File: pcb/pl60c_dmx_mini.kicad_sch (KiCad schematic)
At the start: 36 parts, among them J1 USB-C 16P, J2 XLR-5 female (DMX OUT), Q1 S8050, SW2 BOOT, SW3 USER, U1 ESP32-S3-MINI-1-N8, U2 AP2112K-3.3, U3 SP3485EN, U4 USBLC6-2SC6

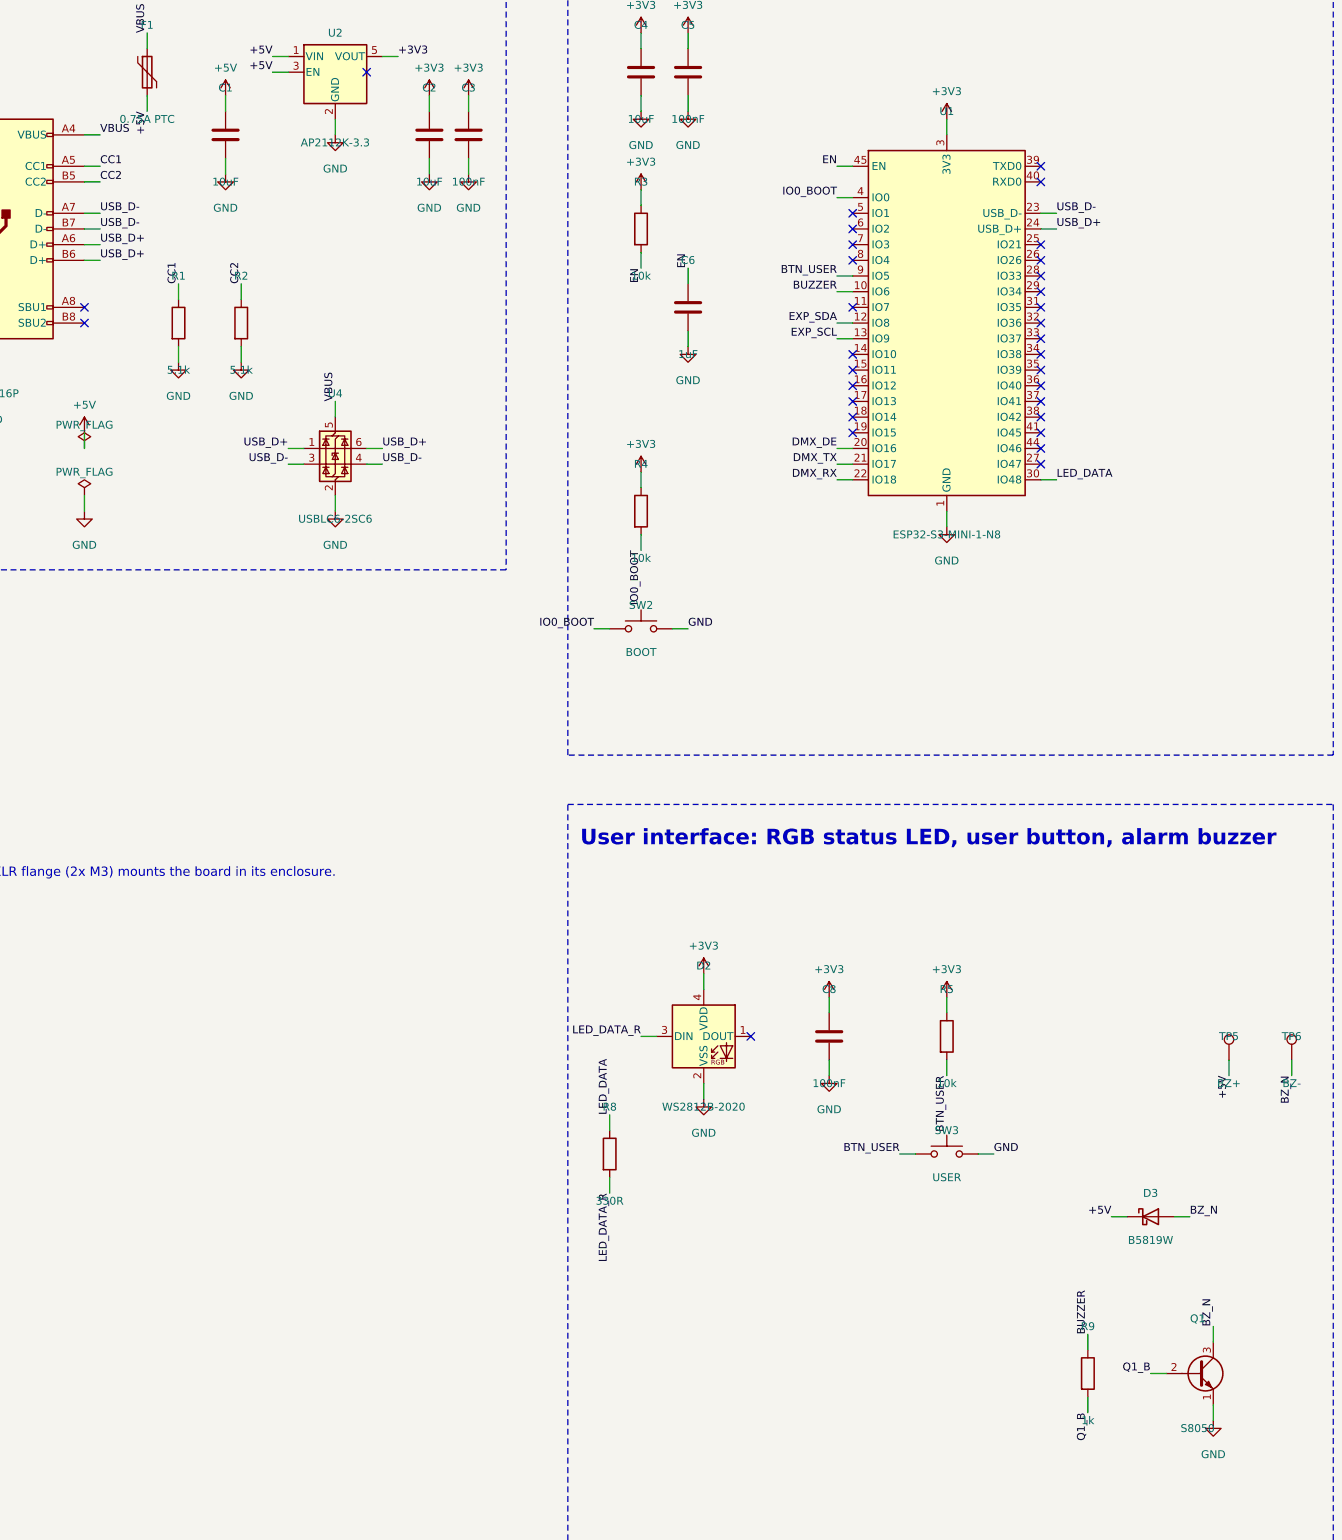
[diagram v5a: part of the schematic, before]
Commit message: auto: 2026-09-02 14:45:57
Co-Authored-By: Claude Fable 5.1 <noreply@anthropic.com>
Claude-Session: https://claude.ai/code/session_01WsrVZb94LwbHVAmBvsSTfn
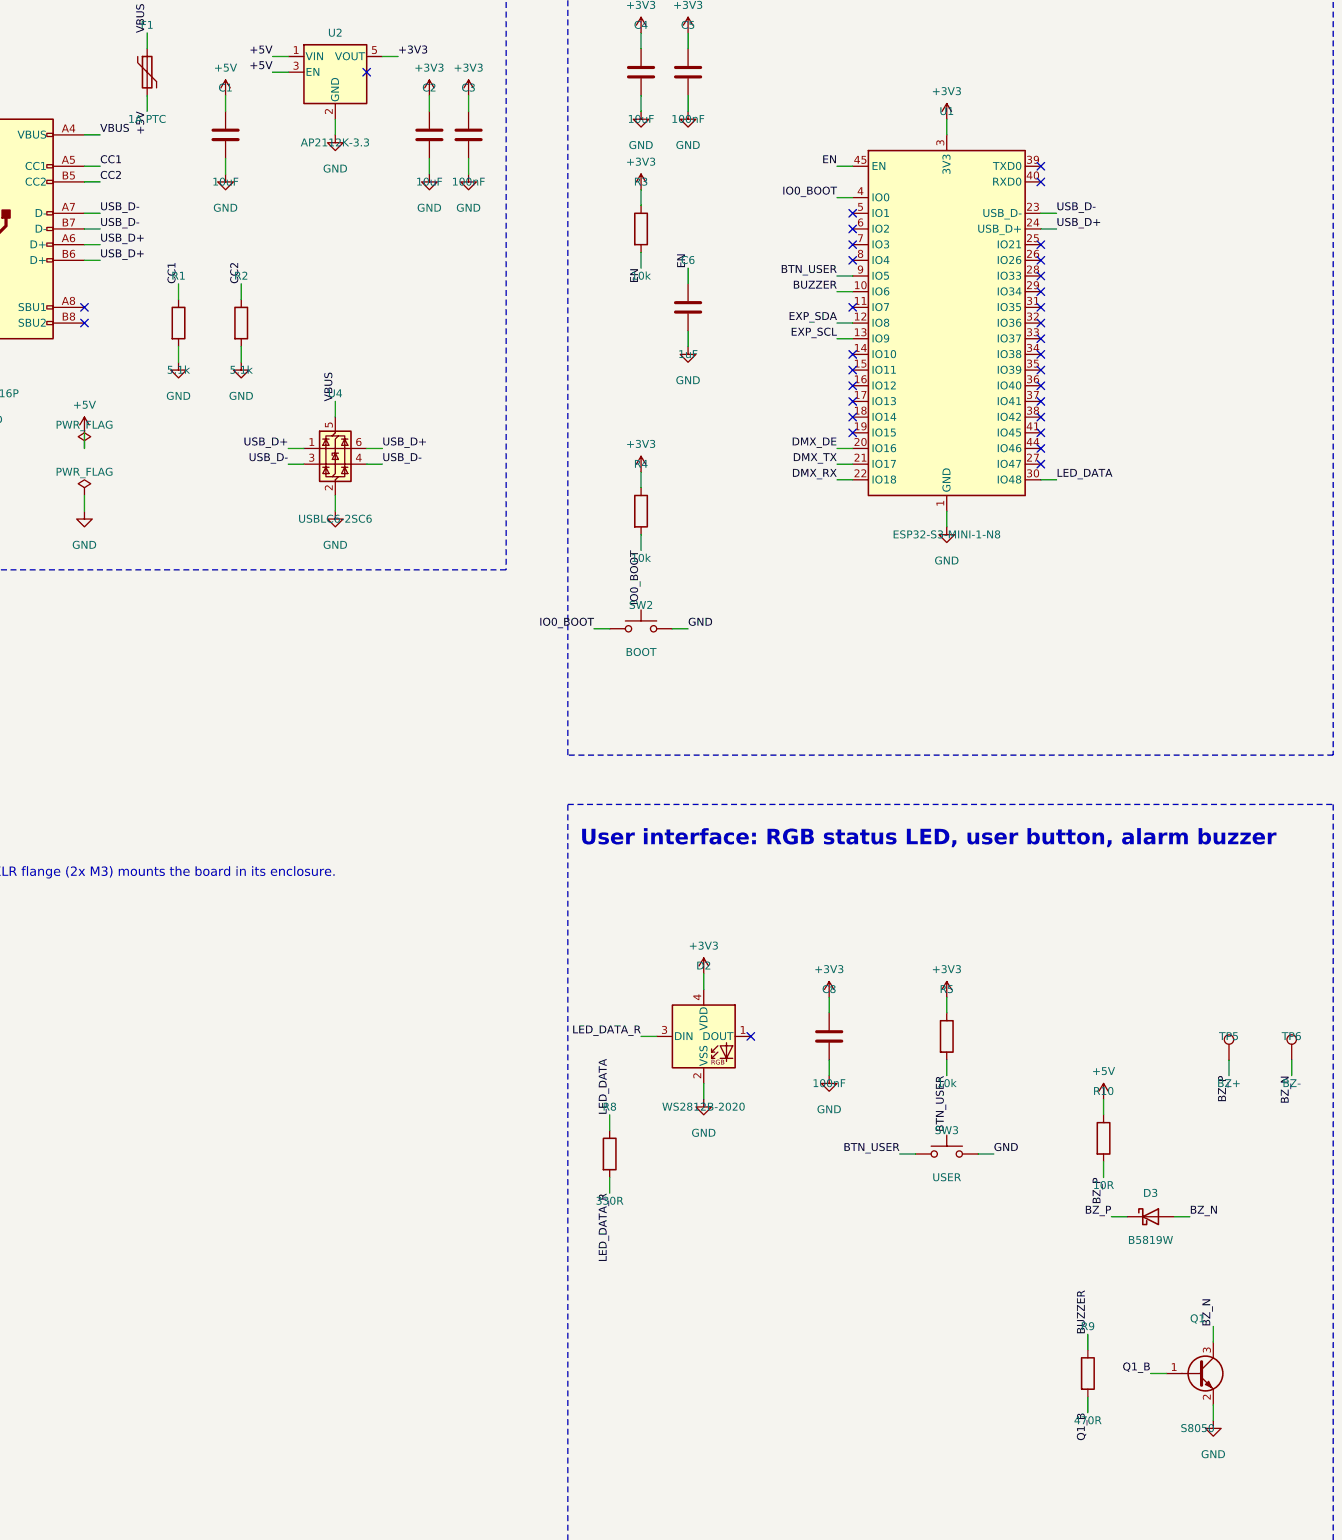
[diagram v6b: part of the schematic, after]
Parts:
- added R10: 10R, Resistor_SMD:R_1206_3216Metric, symbol Device:R
- F1: value 0.75A PTC -> 1A PTC; footprint Fuse:Fuse_0805_2012Metric -> Fuse:Fuse_1206_3216Metric; LCSC C7472571 -> C5358568; MPN 0805L075/6AR -> BSMD1206-100-30V
- Q1: symbol Transistor_BJT:S8050 -> Transistor_BJT:BC817
- R9: value 1k -> 470R; LCSC C11702 -> C25117
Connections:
- net +5V: now also R10.1; no longer D3.1 (K), TP5.1
- net GND: now also Q1.2 (E); no longer Q1.1 (E)
- net Q1_B: now also Q1.1 (B); no longer Q1.2 (B)
- new net BZ_P: D3.1 (K), R10.2, TP5.1
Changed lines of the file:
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@@
 			)
 		)
-		(property "Value" "0.75A PTC"
+		(property "Value" "1A PTC"
 			(at 69.85 46.99 0)
 			(effects
@@
 			)
 		)
-		(property "Footprint" "Fuse:Fuse_0805_2012Metric"
+		(property "Footprint" "Fuse:Fuse_1206_3216Metric"
 			(at 69.85 39.37 0)
 			(effects
@@
 			)
 		)
-		(property "Description" "PTC resettable fuse 0805, 0.75 A hold, 6 V"
+		(property "Description" "PTC resettable fuse 1206, 1 A hold / 1.8 A trip"
 			(at 69.85 39.37 0)
 			(effects
@@
 			)
 		)
-		(property "LCSC" "C7472571"
+		(property "LCSC" "C5358568"
 			(at 69.85 39.37 0)
 			(effects
@@
 			)
 		)
-		(property "MPN" "0805L075/6AR"
+		(property "MPN" "BSMD1206-100-30V"
 			(at 69.85 39.37 0)
 			(effects
@@
 			)
 		)
-		(property "Value" "1k"
+		(property "Value" "470R"
 			(at 222.25 257.81 0)
 			(effects
@@
 			)
 		)
-		(property "Description" "1k 0402"
+		(property "Description" "470R 0402 base resistor"
 			(at 222.25 250.19 0)
 			(effects
@@
 			)
 		)
-		(property "LCSC" "C11702"
+		(property "LCSC" "C25117"
 			(at 222.25 250.19 0)
 			(effects
@@
 	)
 	(symbol
-		(lib_id "Transistor_BJT:S8050")
+		(lib_id "Transistor_BJT:BC817")
 		(at 240.03 250.19 0)
 		(unit 1)
@@
 	(wire
 		(pts
+			(xy 234.95 250.19)
+			(xy 232.41 250.19)
+		)
+		(stroke
+			(width 0)
+			(type default)
+		)
+	)
+	(label "Q1_B"
+		(at 232.41 250.19 180)
+		(fields_autoplaced yes)
+		(effects
+			(font
+				(size 1.27 1.27)
+			)
+			(justify right bottom)
+		)
+	)
+	(wire
+		(pts
 			(xy 242.57 255.27)
 			(xy 242.57 257.81)
@@
 	(wire
 		(pts
-			(xy 234.95 250.19)
-			(xy 232.41 250.19)
-		)
-		(stroke
-			(width 0)
-			(type default)
-		)
-	)
-	(label "Q1_B"
-		(at 232.41 250.19 180)
-		(fields_autoplaced yes)
-		(effects
-			(font
-				(size 1.27 1.27)
-			)
-			(justify right bottom)
-		)
-	)
-	(wire
-		(pts
 			(xy 242.57 245.11)
 			(xy 242.57 242.57)
@@
 		)
 	)
-	(label "+5V"
+	(label "BZ_P"
 		(at 226.06 224.79 180)
 		(fields_autoplaced yes)
@@
 	)
 	(symbol
+		(lib_id "Device:R")
+		(at 224.79 212.09 0)
+		(unit 1)
+		(exclude_from_sim no)
+		(in_bom yes)
+		(on_board yes)
+		(dnp no)
+		(property "Reference" "R10"
+			(at 224.79 204.47 0)
+			(effects
+				(font
+					(size 1.27 1.27)
+				)
+			)
+		)
+		(property "Value" "10R"
+			(at 224.79 219.71 0)
+			(effects
+				(font
+					(size 1.27 1.27)
+				)
+			)
+		)
+		(property "Footprint" "Resistor_SMD:R_1206_3216Metric"
+			(at 224.79 212.09 0)
+			(effects
+				(font
+					(size 1.27 1.27)
+				)
+				(hide yes)
+			)
+		)
+		(property "Datasheet" "~"
+			(at 224.79 212.09 0)
+			(effects
+				(font
+					(size 1.27 1.27)
+				)
+				(hide yes)
+			)
+		)
+		(property "Description" "10R 1206 250mW buzzer series resistor"
+			(at 224.79 212.09 0)
+			(effects
+				(font
+					(size 1.27 1.27)
+				)
+				(hide yes)
+			)
+		)
+		(property "LCSC" "C17903"
+			(at 224.79 212.09 0)
+			(effects
+				(font
+					(size 1.27 1.27)
+				)
+				(hide yes)
+			)
+		)
+		(pin "1"
+		)
+		(pin "2"
+		)
+		(instances
+			(project "pl60c_dmx_mini"
+				(path "/e63f84e3-7254-5f79-8caa-7afae8cc707c"
+					(reference "R10")
+					(unit 1)
+				)
+			)
+		)
+	)
+	(wire
+		(pts
+			(xy 224.79 208.28)
+			(xy 224.79 205.74)
+		)
+		(stroke
+			(width 0)
+			(type default)
+		)
+	)
+	(symbol
+		(lib_id "power:+5V")
+		(at 224.79 205.74 0)
+		(unit 1)
+		(exclude_from_sim no)
+		(in_bom yes)
+		(on_board yes)
+		(dnp no)
+		(property "Reference" "#PWR034"
+			(at 224.79 205.74 0)
+			(effects
+				(font
+					(size 1.27 1.27)
+				)
+				(hide yes)
+			)
+		)
+		(property "Value" "+5V"
+			(at 224.79 201.24 0)
+			(effects
+				(font
+					(size 1.27 1.27)
+				)
+			)
+		)
+		(property "Footprint" ""
+			(at 224.79 205.74 0)
+			(effects
+				(font
+					(size 1.27 1.27)
+				)
+				(hide yes)
+			)
+		)
+		(property "Datasheet" ""
+			(at 224.79 205.74 0)
+			(effects
+				(font
+					(size 1.27 1.27)
+				)
+				(hide yes)
+			)
+		)
+		(property "Description" ""
+			(at 224.79 205.74 0)
+			(effects
+				(font
+					(size 1.27 1.27)
+				)
+				(hide yes)
+			)
+		)
+		(pin "1"
+		)
+		(instances
+			(project "pl60c_dmx_mini"
+				(path "/e63f84e3-7254-5f79-8caa-7afae8cc707c"
+					(reference "#PWR034")
+					(unit 1)
+				)
+			)
+		)
+	)
+	(wire
+		(pts
+			(xy 224.79 215.9)
+			(xy 224.79 218.44)
+		)
+		(stroke
+			(width 0)
+			(type default)
+		)
+	)
+	(label "BZ_P"
+		(at 224.79 218.44 270)
+		(fields_autoplaced yes)
+		(effects
+			(font
+				(size 1.27 1.27)
+			)
+			(justify right bottom)
+		)
+	)
+	(symbol
 		(lib_id "Connector:TestPoint")
 		(at 245.11 199.39 0)
@@
 			)
 		)
-		(property "Description" "External buzzer pad (+5V)"
+		(property "Description" "External buzzer pad (+5V via 10R)"
 			(at 245.11 199.39 0)
 			(effects
@@
 		)
 	)
-	(label "+5V"
+	(label "BZ_P"
 		(at 245.11 201.93 270)
 		(fields_autoplaced yes)
@@
 		(on_board yes)
 		(dnp no)
-		(property "Reference" "#PWR034"
+		(property "Reference" "#PWR035"
 			(at 326.39 193.04 0)
 			(effects
@@
 			(project "pl60c_dmx_mini"
 				(path "/e63f84e3-7254-5f79-8caa-7afae8cc707c"
-					(reference "#PWR034")
+					(reference "#PWR035")
 					(unit 1)
 				)
@@
 		(on_board yes)
 		(dnp no)
-		(property "Reference" "#PWR035"
+		(property "Reference" "#PWR036"
 			(at 59.69 97.79 0)
 			(effects
@@
 			(project "pl60c_dmx_mini"
 				(path "/e63f84e3-7254-5f79-8caa-7afae8cc707c"
-					(reference "#PWR035")
+					(reference "#PWR036")
 					(unit 1)
 				)
@@
 		(on_board yes)
 		(dnp no)
-		(property "Reference" "#FLG036"
+		(property "Reference" "#FLG037"
 			(at 59.69 100.33 0)
 			(effects
@@
 			(project "pl60c_dmx_mini"
 				(path "/e63f84e3-7254-5f79-8caa-7afae8cc707c"
-					(reference "#FLG036")
+					(reference "#FLG037")
 					(unit 1)
 				)
@@
 		(on_board yes)
 		(dnp no)
-		(property "Reference" "#PWR037"
+		(property "Reference" "#PWR038"
 			(at 59.69 110.49 0)
 			(effects
@@
 			(project "pl60c_dmx_mini"
 				(path "/e63f84e3-7254-5f79-8caa-7afae8cc707c"
-					(reference "#PWR037")
+					(reference "#PWR038")
 					(unit 1)
 				)
@@
 		(on_board yes)
 		(dnp no)
-		(property "Reference" "#FLG038"
+		(property "Reference" "#FLG039"
 			(at 59.69 107.95 0)
 			(effects
@@
 			(project "pl60c_dmx_mini"
 				(path "/e63f84e3-7254-5f79-8caa-7afae8cc707c"
-					(reference "#FLG038")
+					(reference "#FLG039")
 					(unit 1)
 				)
